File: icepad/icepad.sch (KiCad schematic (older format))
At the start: 40 parts

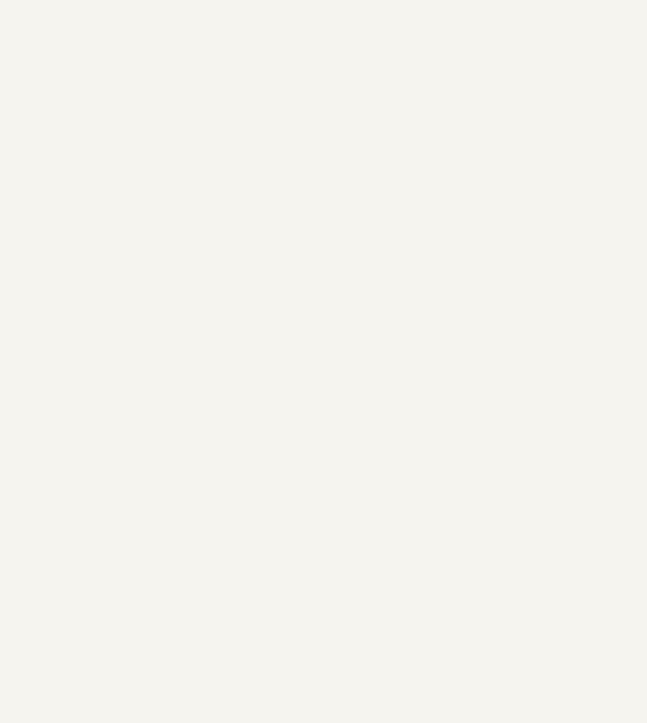
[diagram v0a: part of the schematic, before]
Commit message: added mcu
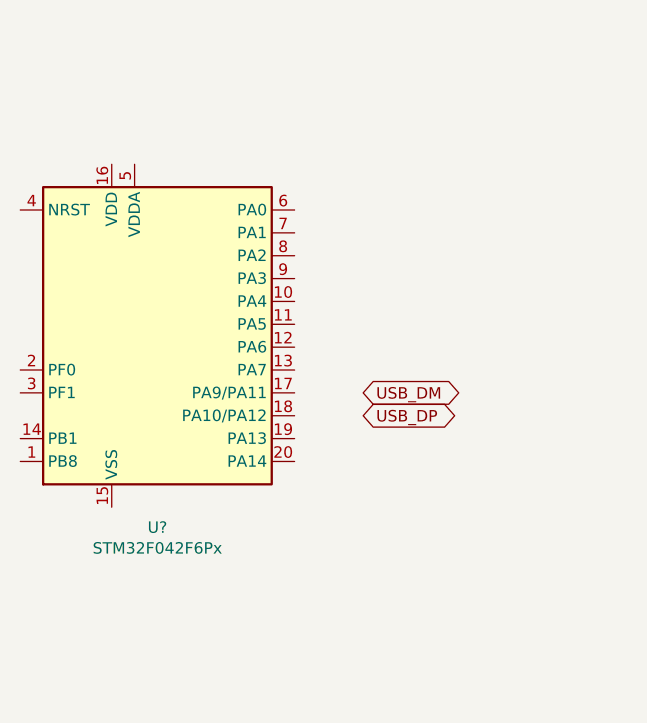
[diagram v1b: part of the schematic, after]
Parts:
- added U?: STM32F042F6Px, Package_SO:TSSOP-20_4.4x6.5mm_P0.65mm, symbol MCU_ST_STM32F0:STM32F042F6Px
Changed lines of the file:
@@
 EESchema Schematic File Version 4
+LIBS:icepad-cache
 EELAYER 30 0
 EELAYER END
@@
 	1    0    0    -1
 $EndComp
+$Comp
+L MCU_ST_STM32F0:STM32F042F6Px U?
+U 1 1 5E43D887
+P 3600 3000
+F 0 "U?" H 3600 2111 50  0000 C CNN
+F 1 "STM32F042F6Px" H 3600 2020 50  0000 C CNN
+F 2 "Package_SO:TSSOP-20_4.4x6.5mm_P0.65mm" H 3100 2300 50  0001 R CNN
+F 3 "http://www.st.com/st-web-ui/static/active/en/resource/technical/document/datasheet/DM00105814.pdf" H 3600 3000 50  0001 C CNN
+	1    3600 3000
+	1    0    0    -1
+$EndComp
+Text GLabel 4500 3300 2    50   BiDi ~ 0
+USB_DM
+Text GLabel 4500 3400 2    50   BiDi ~ 0
+USB_DP
 $EndSCHEMATC
